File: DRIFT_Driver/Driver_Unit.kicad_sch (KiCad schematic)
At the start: 28 parts, among them IC1 DRV8313RHHR, U1 INA199xxDCK, U2 74HC32

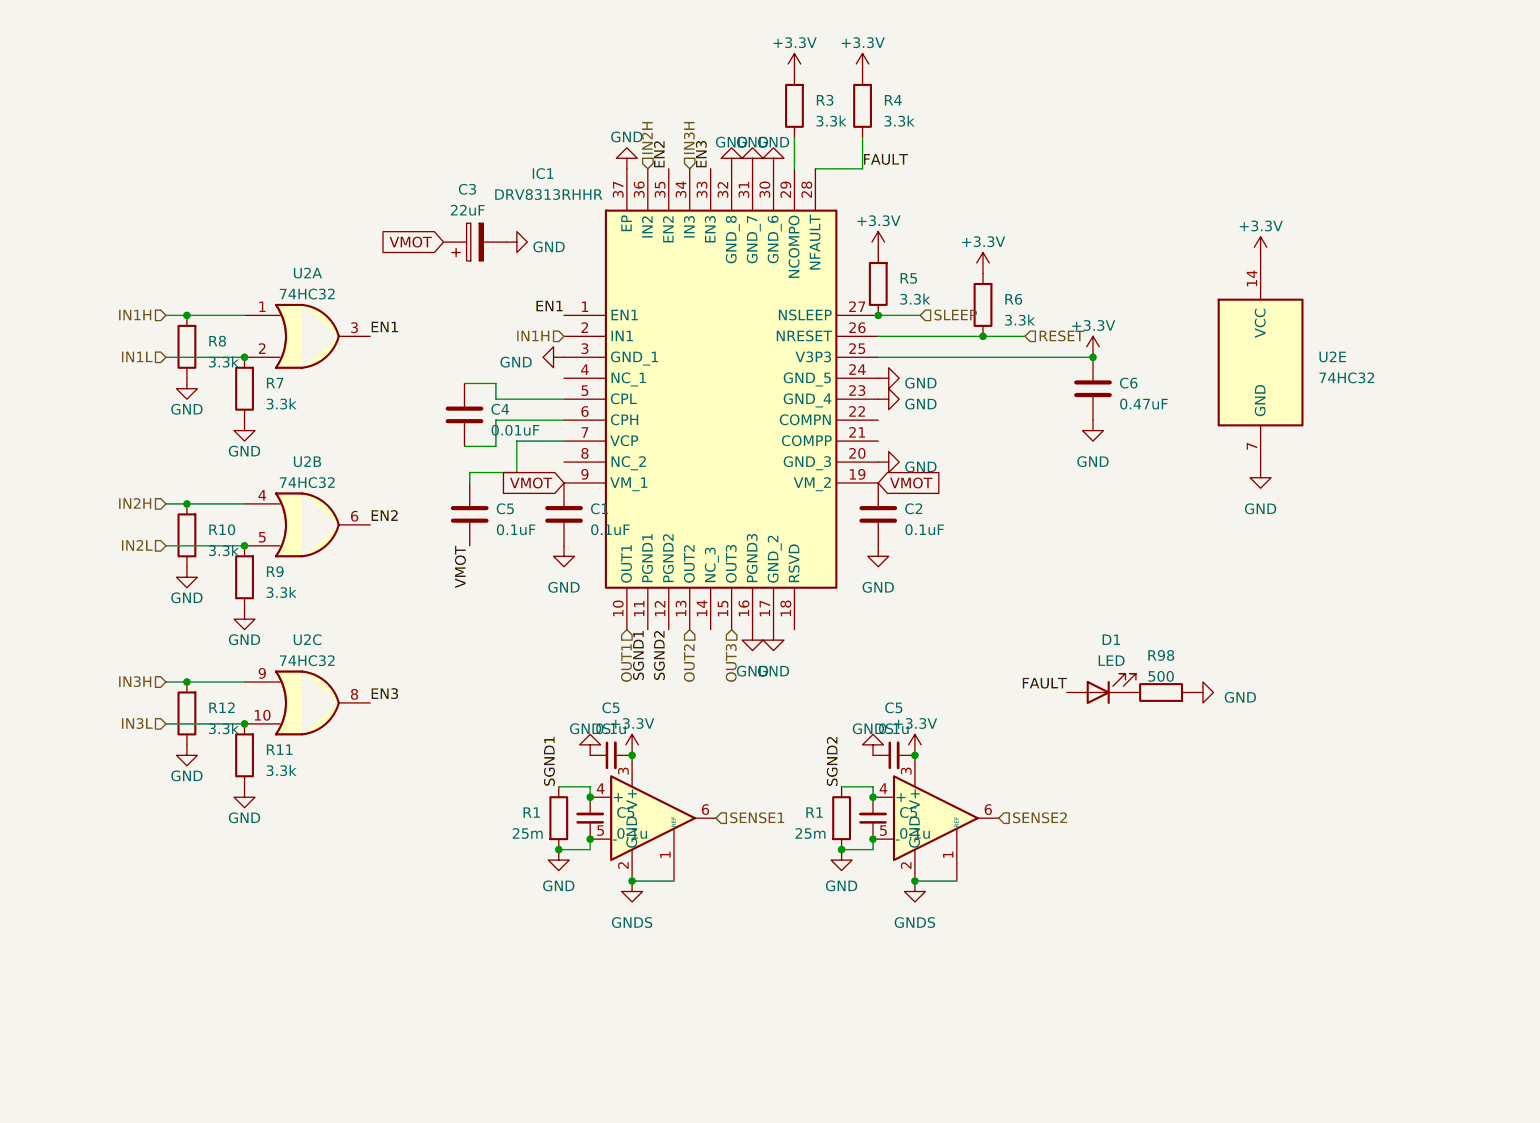
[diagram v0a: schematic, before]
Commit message: Finished majority of component implementations
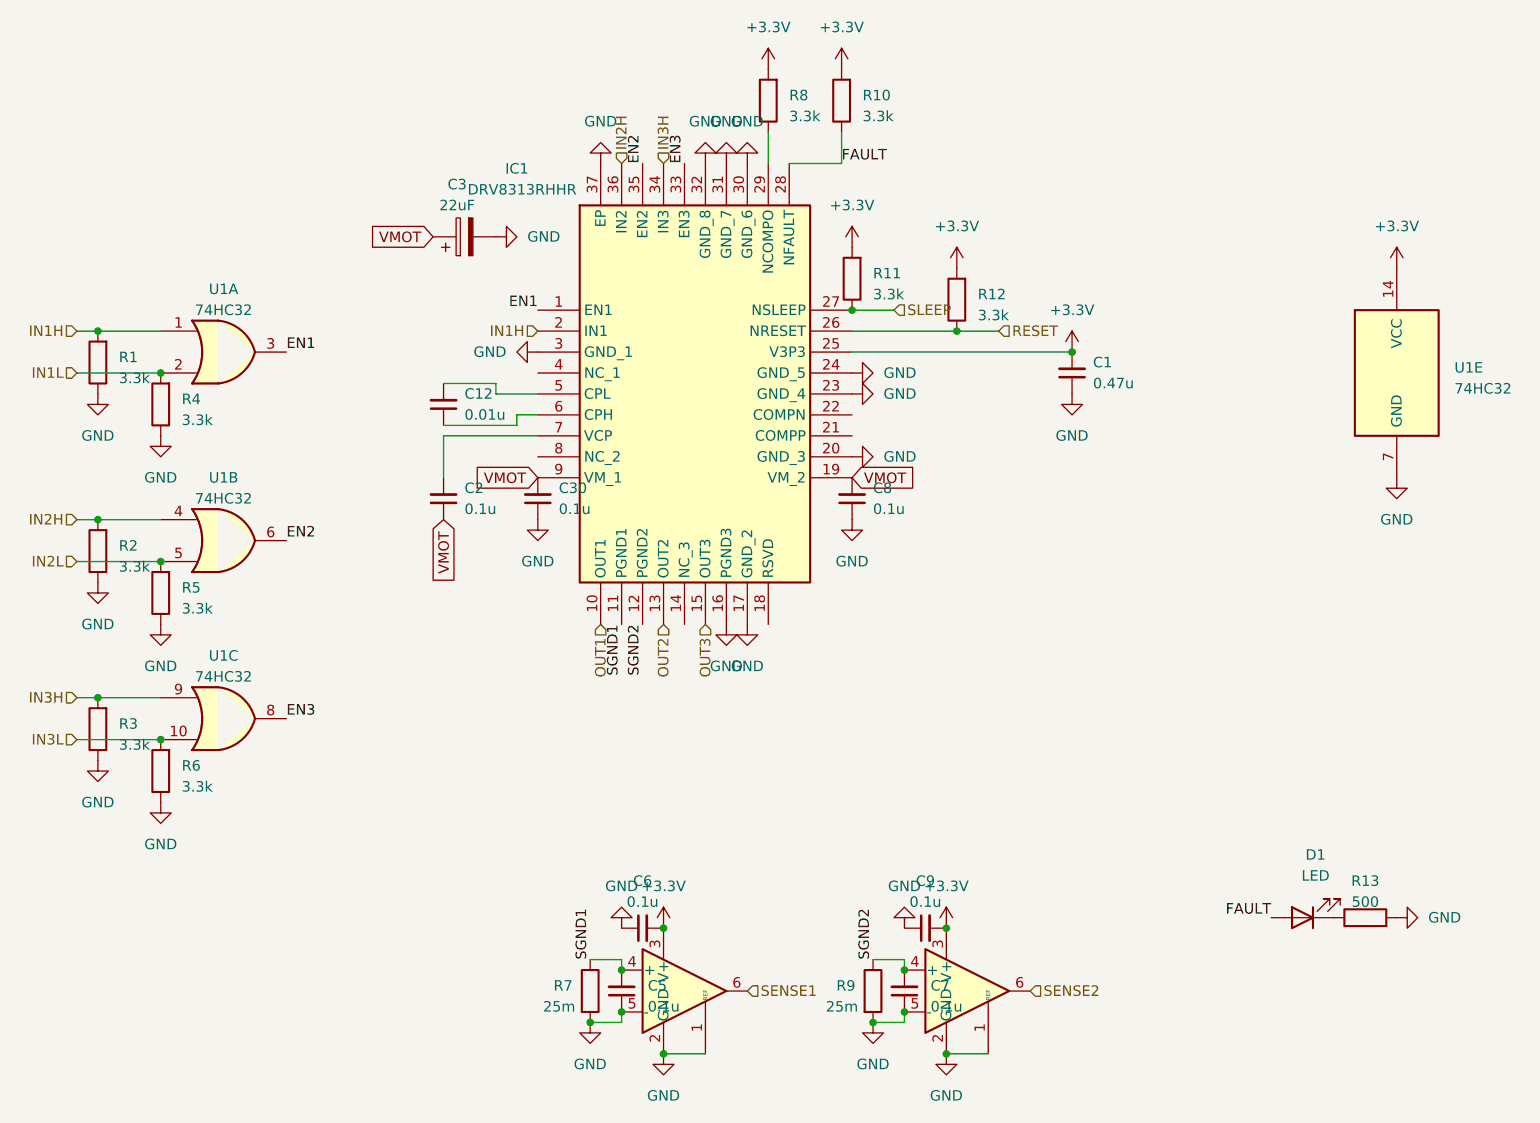
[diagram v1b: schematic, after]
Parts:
- removed C1, C2, C5: 0.1uF, symbol Device:C
- removed C4: 0.01uF, symbol Device:C
- removed C6: 0.47uF, symbol Device:C
- added C1: 0.47u, Capacitor_SMD:C_0402_1005Metric, symbol Device:C_Small
- added C12: 0.01u, Capacitor_SMD:C_0402_1005Metric, symbol Device:C_Small
- added C2, C30, C8: 0.1u, Capacitor_SMD:C_0402_1005Metric, symbol Device:C_Small
- C3: footprint (none) -> Capacitor_SMD:C_0402_1005Metric
- IC1: footprint QFN50P600X600X100-37N-D -> Touchstone:QFN50P600X600X100-37N-D
- R1: renamed from R8; footprint (none) -> Resistor_SMD:R_0402_1005Metric
- R10: renamed from R4; footprint (none) -> Resistor_SMD:R_0402_1005Metric
- R11: renamed from R5; footprint (none) -> Resistor_SMD:R_0402_1005Metric
- R12: renamed from R6; footprint (none) -> Resistor_SMD:R_0402_1005Metric
- R2: renamed from R10; footprint (none) -> Resistor_SMD:R_0402_1005Metric
- R3: renamed from R12; footprint (none) -> Resistor_SMD:R_0402_1005Metric
- R4: renamed from R7; footprint (none) -> Resistor_SMD:R_0402_1005Metric
- R5: renamed from R9; footprint (none) -> Resistor_SMD:R_0402_1005Metric
- R6: renamed from R11; footprint (none) -> Resistor_SMD:R_0402_1005Metric
- R8: renamed from R3; footprint (none) -> Resistor_SMD:R_0402_1005Metric
- U1: renamed from U2; footprint (none) -> Package_SO:SOIC-14_3.9x8.7mm_P1.27mm
- renumbered C5 to C6, C5 to C7, C5 to C9, R98 to R13, R1 to R7, R1 to R9, U1 to U2, U1 to U3
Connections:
- net GNDS is gone; now on net GND: C6.1, C9.1, U2.1 (REF), U2.2 (GND), U3.1 (REF), U3.2 (GND)
- net +3.3V: now also C1.2
- net GND: now also C1.1, C30.1, C8.1
- net VMOT: now also C2.1, C30.2, C8.2
- net at IC1.5 (CPL): now also C12.2
- net at IC1.6 (CPH): now also C12.1
- net at IC1.7 (VCP): now also C2.2
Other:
- moved on the sheet: C3, C5, C6, C7, C9, IC1, R1, R10, R11, R12, R13, R2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
